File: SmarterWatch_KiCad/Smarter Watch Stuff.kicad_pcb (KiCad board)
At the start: 4 copper layers, 39 x 39 mm, 111 parts, among them J5 CX70M-24P1, M1 Motor_DC, Q1 2N7002, Q2 2N7002, Q3 2N7002, Q4 2N7002, SW1 SW_SPST, SW2 SW_SPST, U1 MCP7940N-xSN, U10 MAX30102, U11 BMI160, U15 M24C64-WMN6TP, U16 IQS323001DNR, U17 MAX30205MTA+T, U2 TSL25911FN, U21 MMC5983MA, U24 AS3935-BQFT, U25 SGP40-D-R4, U26 NLA9306MU3TAG, U3 MCP73831-2-MC, U4 TCR2EE10, U5 ESP32-C6-MINI-1, U6 SHTC3, U7 TMP117xxDRV, U8 ST7735, U9 MIC5365-1.8YC5, Y1 Crystal

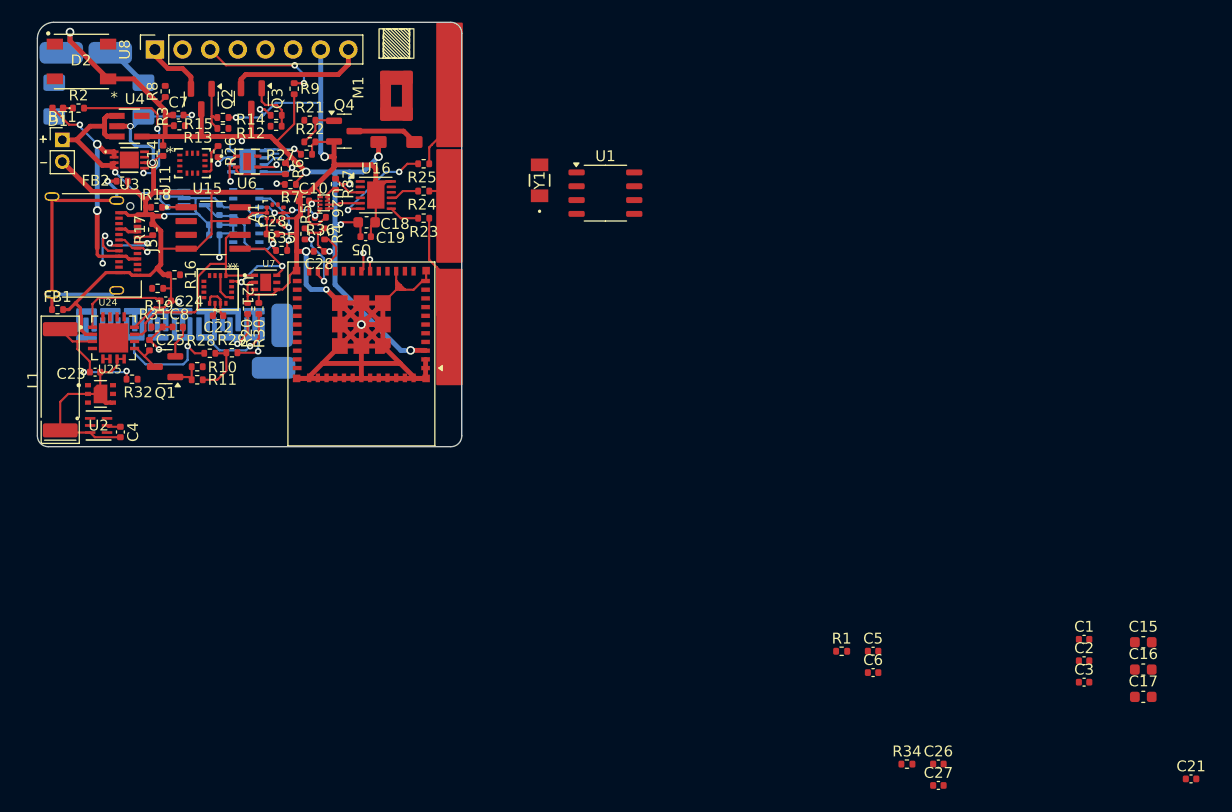
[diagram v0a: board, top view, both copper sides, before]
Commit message: Routing!
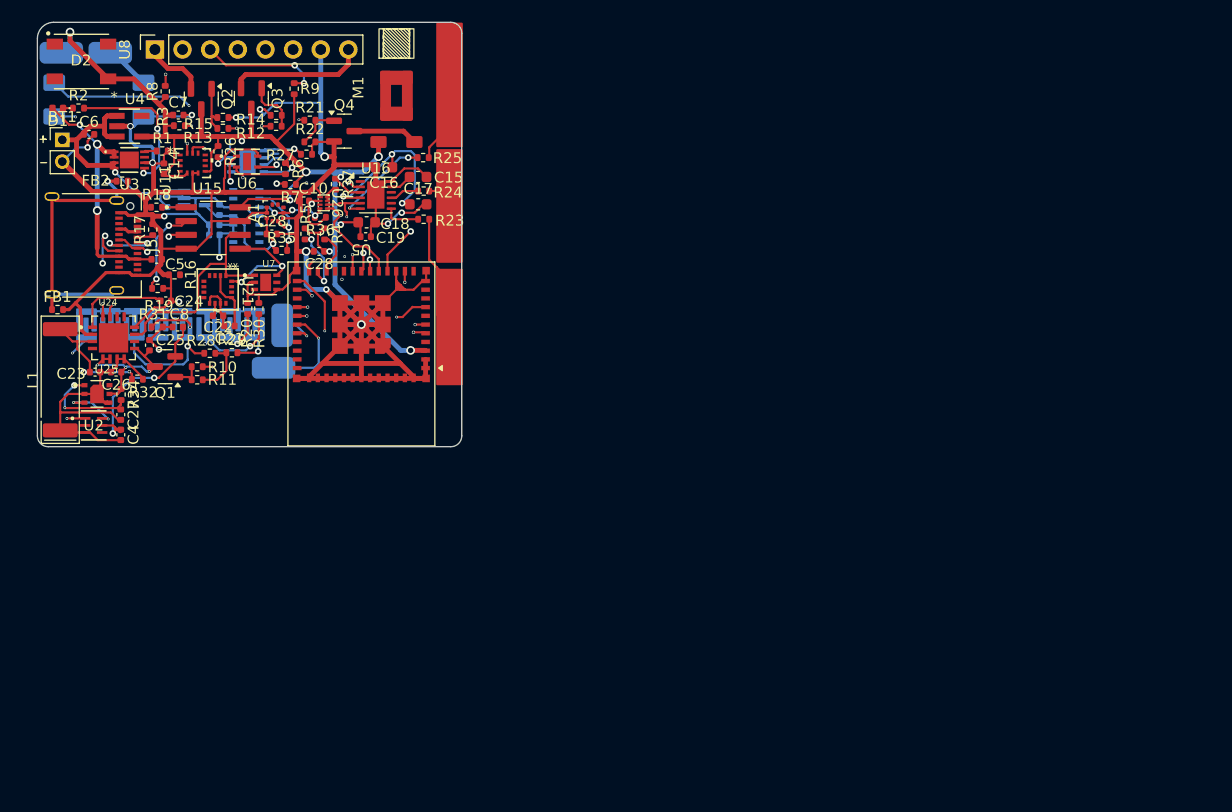
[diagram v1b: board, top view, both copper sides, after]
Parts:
- removed C1: 1 uf, Capacitor_SMD:C_0402_1005Metric
- removed C2, C3: 12 picoF, Capacitor_SMD:C_0402_1005Metric
- removed U1: MCP7940N-xSN, Package_SO:JEITA_SOIC-8_3.9x4.9mm_P1.27mm
- removed Y1: Crystal, Custom_Foot:XTAL_SC32S-7PF20PPM_EPS
- moved C21 97.7 mm to (87.1, 68.4), turned to 180 degrees
- moved C6 87.4 mm to (74.2, 50.8)
- moved C26 83.7 mm to (76.7, 72.6), turned to 180 degrees
- moved C16 83.7 mm to (101.3, 53.8), turned to 180 degrees
- moved C27 82.5 mm to (77.2, 76.6), turned to -90 degrees
- moved C17 80.6 mm to (104.5, 57.2)
- moved R34 79.8 mm to (77.2, 74.7), turned to -90 degrees
- moved C15 79.2 mm to (104.5, 54.7)
- moved R1 77.5 mm to (81.0, 52.3)
- moved C5 75.0 mm to (80.5, 62.3), turned to 180 degrees
- moved C14 1.65 mm to (81.1, 53.9), turned to -90 degrees
- moved R25 0.57 mm to (105.0, 52.9)
- moved R32 0.49 mm to (78.7, 73.3)
- moved U2 0.45 mm to (74.7, 77.5)
- moved U25 0.32 mm to (75.0, 74.7)
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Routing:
- net Net-(SW1-B): track 0.00 -> 52.4 mm, vias 0 -> 3
- net +3.3V: track 108.1 -> 148.7 mm, vias 9 -> 13
- net Screen_Reset: track 0.00 -> 39.1 mm, vias 0 -> 1
- net Screen_A0: track 0.00 -> 38.4 mm, vias 0 -> 1
- net SDA: track 15.5 -> 53.1 mm, vias 4 -> 9
- net Screen_CS: track 0.00 -> 35.2 mm, vias 0 -> 1
- net SCLK: track 0.00 -> 34.1 mm, vias 0 -> 2
- net GND: track 323.9 -> 357.3 mm, vias 12 -> 15
- net MOSI: track 11.3 -> 39.8 mm, vias 2 -> 3
- net Backlight: track 0.00 -> 25.0 mm, vias 0 -> 4
- net Vibrate: track 0.00 -> 22.3 mm, vias 0 -> 3
- net Net-(U15-A1): track 0.00 -> 21.5 mm, vias 0 -> 3
- net SCL: track 28.3 -> 49.5 mm, vias 0 -> 5
- net Sensor_enable: track 0.00 -> 18.6 mm, vias 0 -> 2
- net Screen_power: track 0.00 -> 18.2 mm, vias 0 -> 2
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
